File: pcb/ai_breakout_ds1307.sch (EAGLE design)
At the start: 11 parts, among them J2 1X06, U1 DS1307SO8

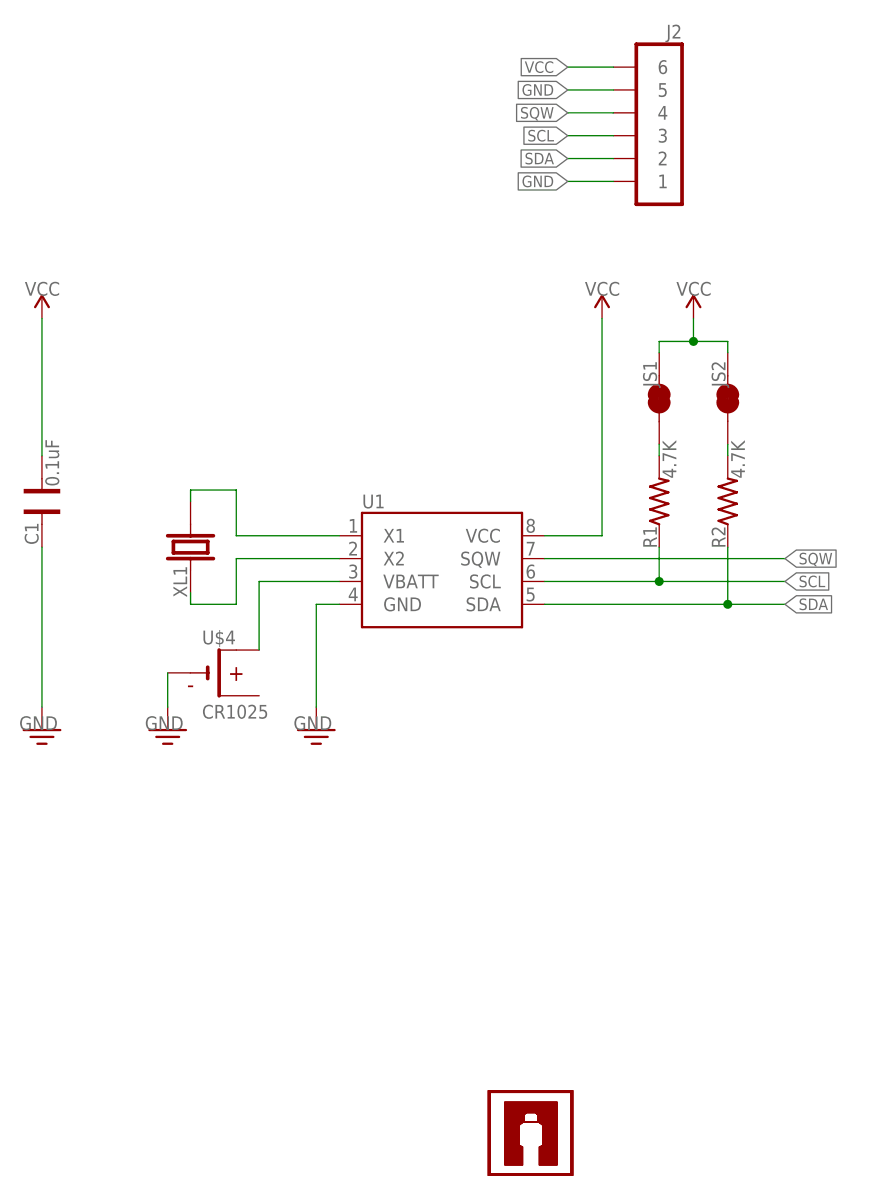
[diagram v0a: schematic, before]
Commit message: board updated
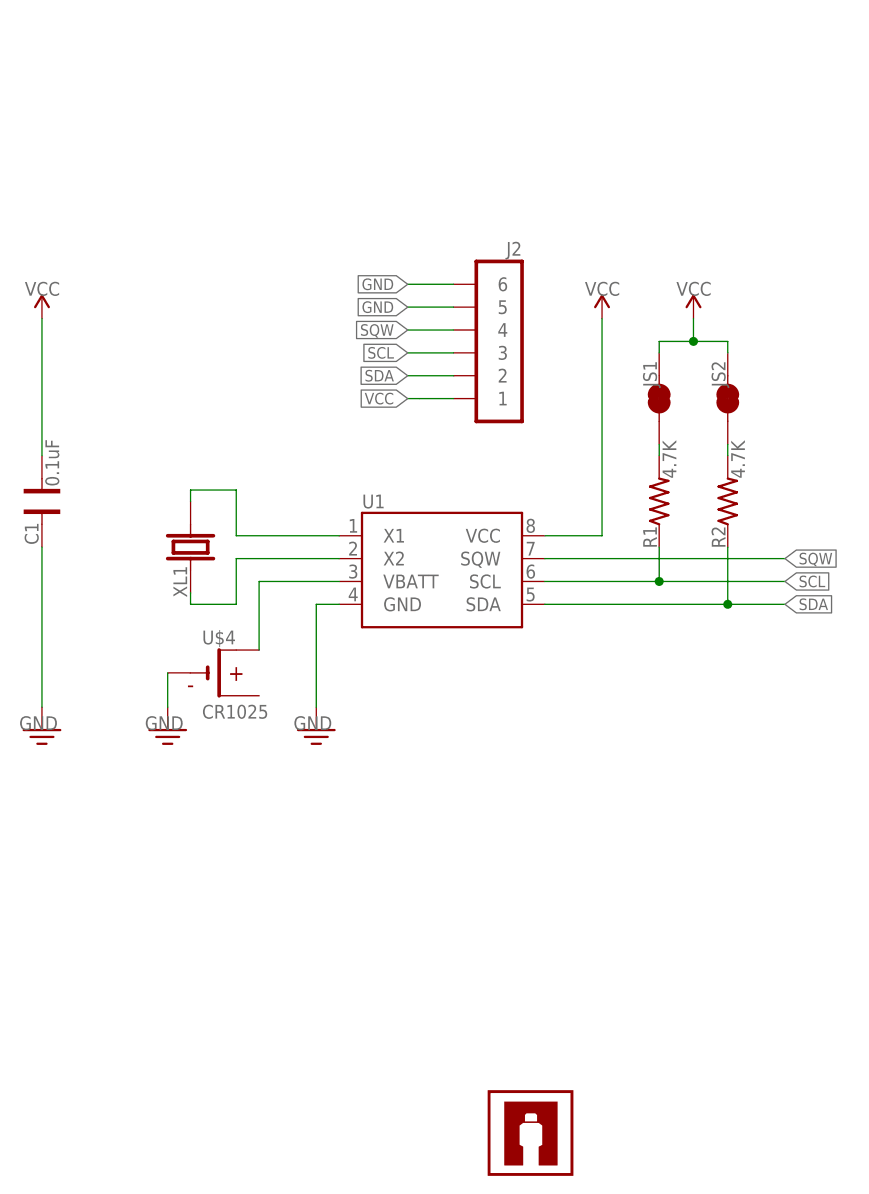
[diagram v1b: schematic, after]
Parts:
- removed U$2: AI-LOGOXS, Ai_Miscellany:AI-LOGOXS
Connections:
- net GND: now also J2.6; no longer J2.1
- net VCC: now also J2.1; no longer J2.6
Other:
- moved on the sheet: J2
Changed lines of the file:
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@@
 <part name="C1" library="Ai_Passives" deviceset="CAP" device="0603" value="0.1uF"/>
 <part name="GND2" library="Ai_Power" deviceset="GND" device=""/>
-<part name="U$2" library="Ai_Miscellany" deviceset="AI-LOGO" device="XS"/>
 <part name="U$3" library="Ai_Miscellany" deviceset="AI-LOGO" device="XS"/>
 <part name="U$4" library="Ai_Connectors" deviceset="CR1025" device=""/>
@@
 <instance part="R2" gate="G$1" x="158.75" y="82.55" rot="R90"/>
 <instance part="VCC2" gate="1" x="154.94" y="102.87"/>
-<instance part="J2" gate="M06X1" x="151.13" y="125.73" rot="MR0"/>
+<instance part="J2" gate="M06X1" x="133.35" y="101.6" rot="MR0"/>
 <instance part="GND1" gate="GND" x="113.03" y="57.15"/>
 <instance part="VCC3" gate="1" x="82.55" y="102.87"/>
 <instance part="C1" gate="G$1" x="82.55" y="82.55"/>
 <instance part="GND2" gate="GND" x="82.55" y="57.15"/>
-<instance part="U$2" gate="G$1" x="132.08" y="7.62"/>
 <instance part="U$3" gate="G$1" x="132.08" y="7.62"/>
 <instance part="U$4" gate="G$1" x="101.6" y="63.5"/>
@@
 </segment>
 <segment>
-<pinref part="J2" gate="M06X1" pin="6"/>
-<wire x1="146.05" y1="130.81" x2="140.97" y2="130.81" width="0.1524" layer="91"/>
-<label x="140.97" y="130.81" size="1.27" layer="95" font="vector" ratio="10" rot="R180" xref="yes"/>
+<pinref part="J2" gate="M06X1" pin="1"/>
+<wire x1="128.27" y1="93.98" x2="124.46" y2="93.98" width="0.1524" layer="91"/>
+<wire x1="123.19" y1="93.98" x2="124.46" y2="93.98" width="0.1524" layer="91"/>
+<label x="123.19" y="93.98" size="1.27" layer="95" font="vector" ratio="10" rot="R180" xref="yes"/>
 </segment>
 </net>
@@
 <segment>
 <pinref part="J2" gate="M06X1" pin="4"/>
-<wire x1="146.05" y1="125.73" x2="140.97" y2="125.73" width="0.1524" layer="91"/>
-<label x="140.97" y="125.73" size="1.27" layer="95" font="vector" ratio="10" rot="R180" xref="yes"/>
+<wire x1="128.27" y1="101.6" x2="123.19" y2="101.6" width="0.1524" layer="91"/>
+<label x="123.19" y="101.6" size="1.27" layer="95" font="vector" ratio="10" rot="R180" xref="yes"/>
 </segment>
 </net>
@@
 <segment>
 <pinref part="J2" gate="M06X1" pin="3"/>
-<wire x1="146.05" y1="123.19" x2="140.97" y2="123.19" width="0.1524" layer="91"/>
-<label x="140.97" y="123.19" size="1.27" layer="95" font="vector" ratio="10" rot="R180" xref="yes"/>
+<wire x1="128.27" y1="99.06" x2="123.19" y2="99.06" width="0.1524" layer="91"/>
+<label x="123.19" y="99.06" size="1.27" layer="95" font="vector" ratio="10" rot="R180" xref="yes"/>
 </segment>
 </net>
@@
 <segment>
 <pinref part="J2" gate="M06X1" pin="2"/>
-<wire x1="146.05" y1="120.65" x2="140.97" y2="120.65" width="0.1524" layer="91"/>
-<label x="140.97" y="120.65" size="1.27" layer="95" font="vector" ratio="10" rot="R180" xref="yes"/>
+<wire x1="128.27" y1="96.52" x2="123.19" y2="96.52" width="0.1524" layer="91"/>
+<label x="123.19" y="96.52" size="1.27" layer="95" font="vector" ratio="10" rot="R180" xref="yes"/>
 </segment>
 </net>
@@
 <segment>
 <pinref part="J2" gate="M06X1" pin="5"/>
-<wire x1="146.05" y1="128.27" x2="140.97" y2="128.27" width="0.1524" layer="91"/>
-<label x="140.97" y="128.27" size="1.27" layer="95" font="vector" ratio="10" rot="R180" xref="yes"/>
-</segment>
-<segment>
-<pinref part="J2" gate="M06X1" pin="1"/>
-<wire x1="146.05" y1="118.11" x2="140.97" y2="118.11" width="0.1524" layer="91"/>
-<label x="140.97" y="118.11" size="1.27" layer="95" font="vector" ratio="10" rot="R180" xref="yes"/>
+<wire x1="128.27" y1="104.14" x2="123.19" y2="104.14" width="0.1524" layer="91"/>
+<label x="123.19" y="104.14" size="1.27" layer="95" font="vector" ratio="10" rot="R180" xref="yes"/>
 </segment>
 <segment>
@@
 <pinref part="GND3" gate="GND" pin="GND"/>
 </segment>
+<segment>
+<pinref part="J2" gate="M06X1" pin="6"/>
+<wire x1="128.27" y1="106.68" x2="123.19" y2="106.68" width="0.1524" layer="91"/>
+<label x="123.19" y="106.68" size="1.27" layer="95" font="vector" ratio="10" rot="R180" xref="yes"/>
+</segment>
 </net>
